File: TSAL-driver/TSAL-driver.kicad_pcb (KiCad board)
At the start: 2 copper layers, 20.3 x 56.5 mm, 12 parts, among them J1 LED+, J2 LED-, J3 12V, J4 GND, U1 AZ1117-5.0, U2 ATtiny25-20SSU, U3 LDB-350L

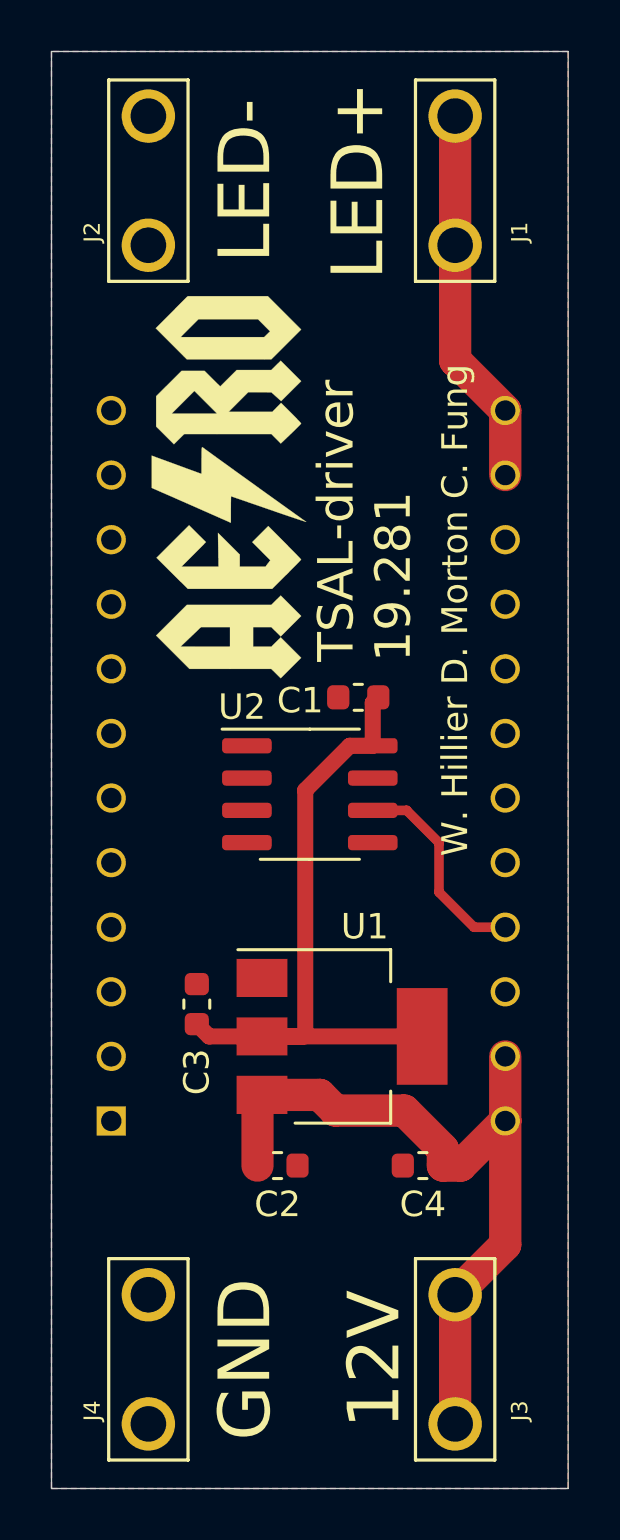
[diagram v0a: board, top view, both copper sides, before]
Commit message: Cleaned up board, added 3D
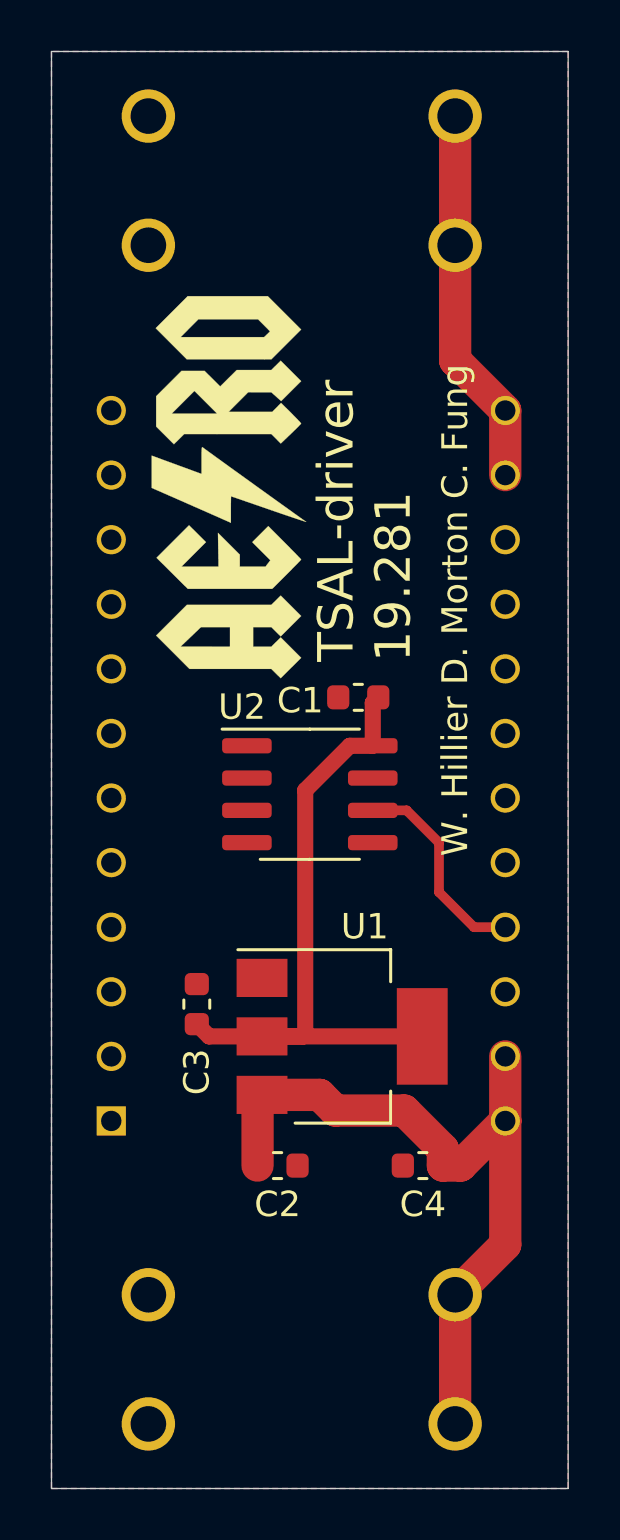
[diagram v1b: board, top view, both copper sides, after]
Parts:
- J1, J2, J3, J4: moved to B.Cu
- turned J1 to 270 degrees
- turned J2 to 270 degrees
- turned J3 to 270 degrees
- turned J4 to 270 degrees
